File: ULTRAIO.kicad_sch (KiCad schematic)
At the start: 8 parts, among them U6 FDC37C932FR_1.3

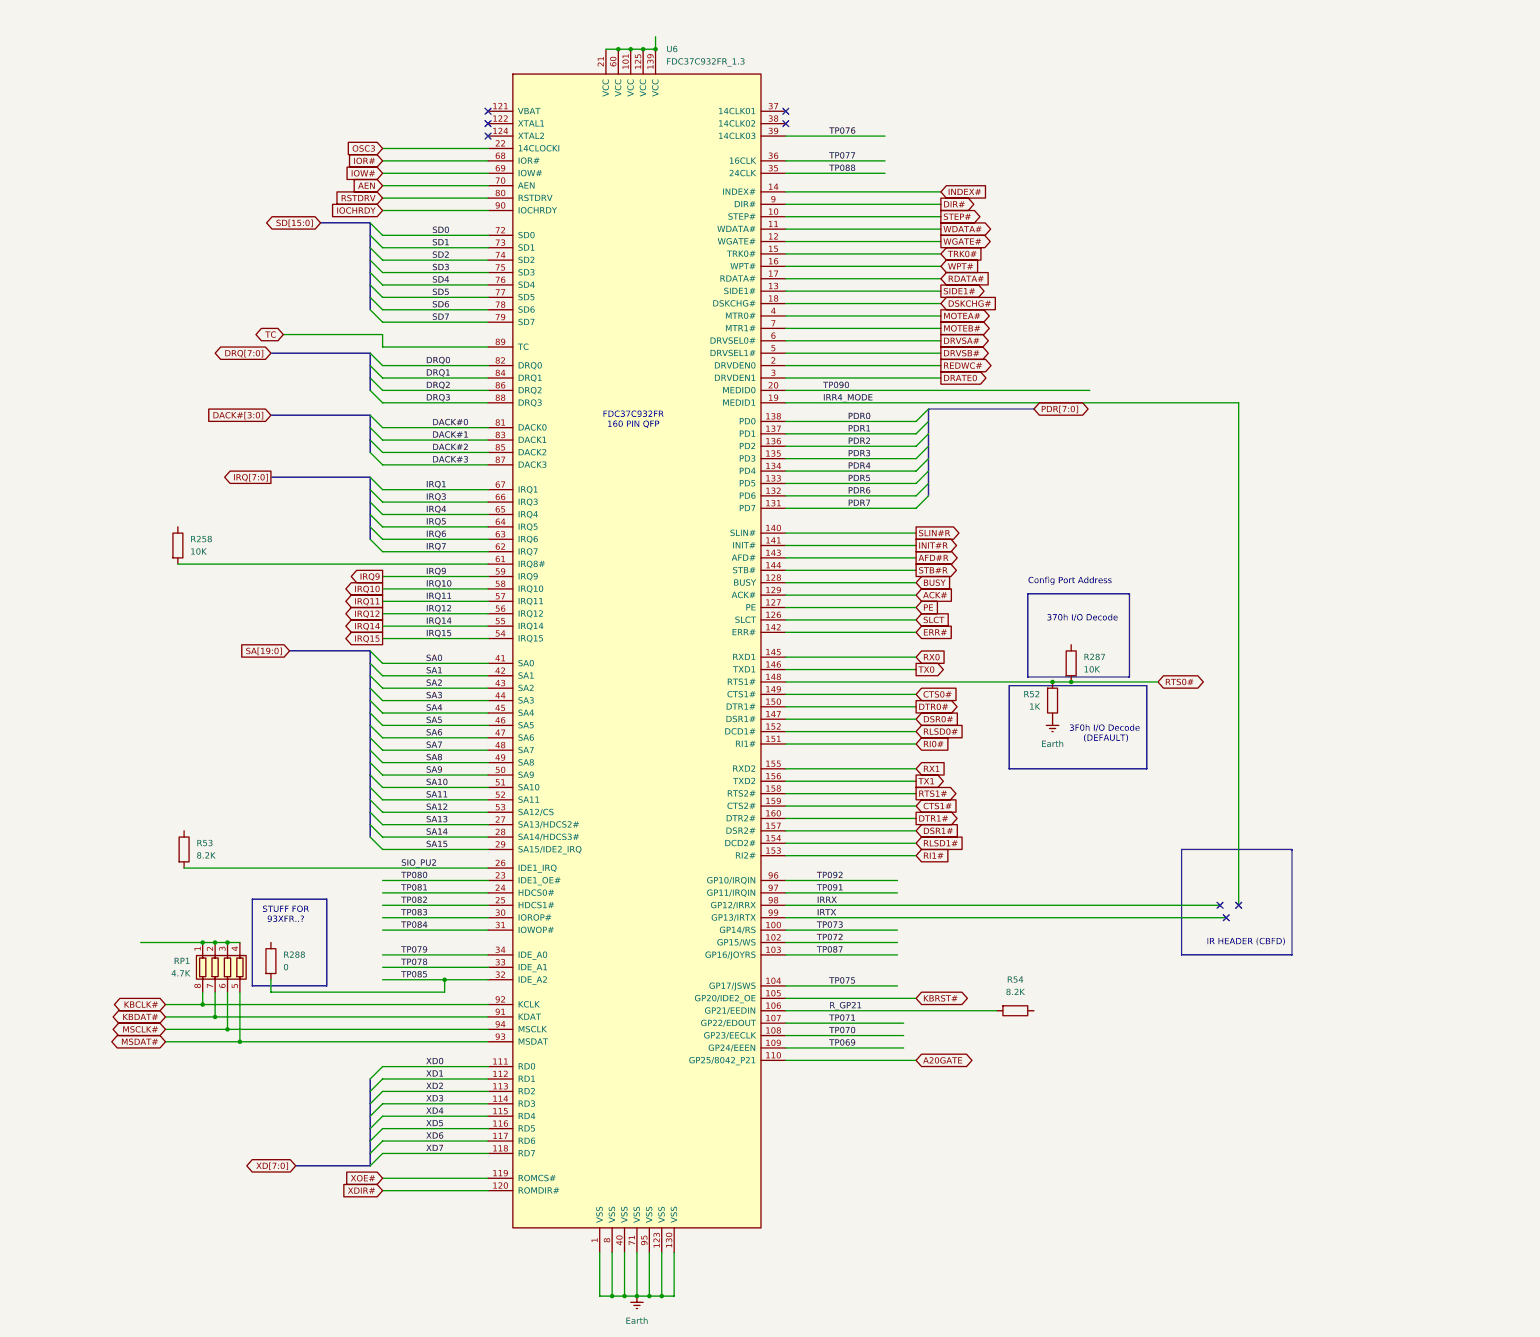
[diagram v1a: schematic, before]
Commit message: ULTRA I/O page 14
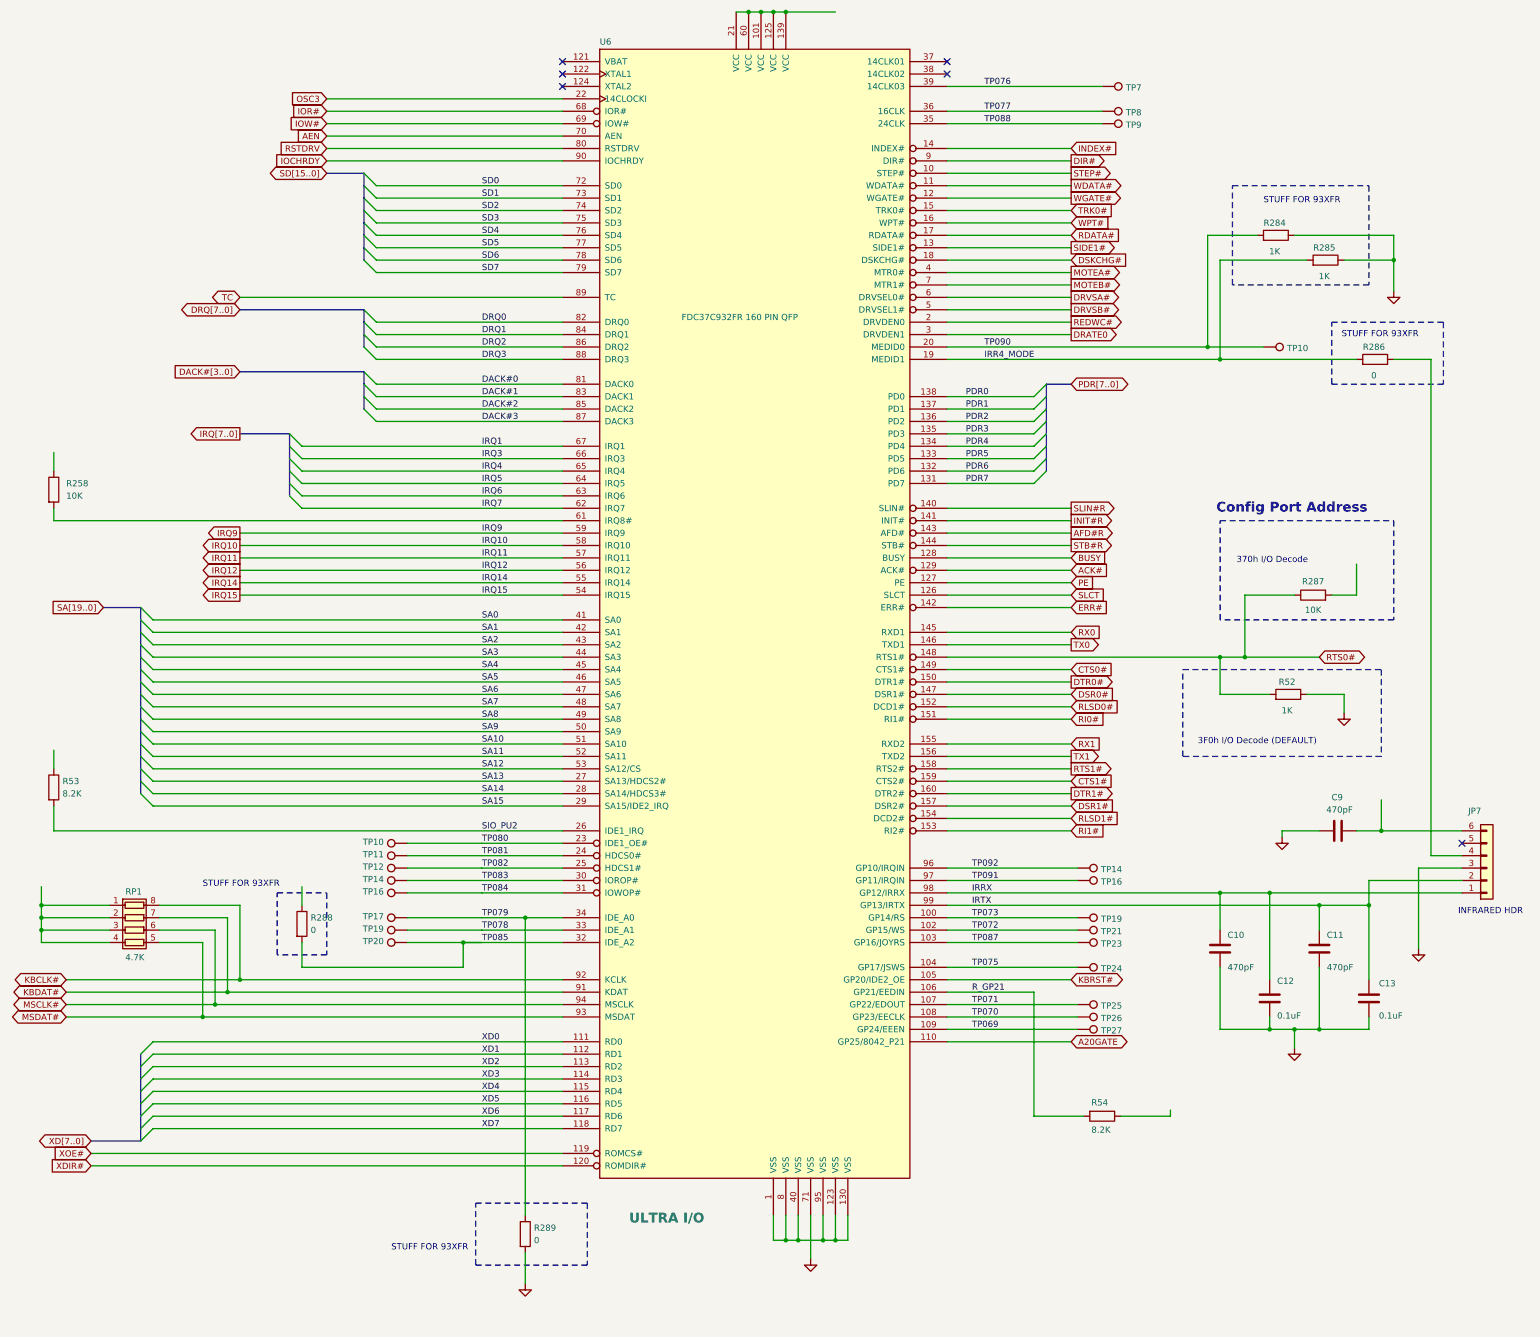
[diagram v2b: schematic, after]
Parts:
- added C10, C11, C9: 470pF, Capacitor_SMD:C_0201_0603Metric, symbol Device:C
- added C12, C13: 0.1uF, Capacitor_SMD:C_0201_0603Metric, symbol Device:C
- added JP7: Conn_01x06, symbol Connector_Generic:Conn_01x06
- added R284, R285: 1K, Resistor_SMD:R_0201_0603Metric, symbol Device:R
- added R286, R289: 0, Resistor_SMD:R_0201_0603Metric, symbol Device:R
- added TP10 (x2), TP11, TP12, TP14 (x2), TP16 (x2), TP17, TP19 (x2), TP20, TP21, TP23, TP24, TP25, TP26, TP27, TP7, TP8, TP9: TestPoint, symbol Connector:TestPoint
- U6: value FDC37C932FR_1.3 -> FDC37C932FR 160 PIN QFP
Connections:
- net IRR4_MODE: now also R285.2, R286.2
- net IRRX: now also C10.1, C12.1, JP7.1 (Pin_1)
- net IRTX: now also C11.1, C13.1, JP7.2 (Pin_2)
- net RTS0#: now also R287.1; no longer R287.2
- net TP069: now also TP27.1
- net TP070: now also TP26.1
- net TP071: now also TP25.1
- net TP072: now also TP21.1
- net TP073: now also TP19.1
- net TP075: now also TP24.1
- net TP076: now also TP7.1
- net TP077: now also TP8.1
- net TP078: now also TP19.1
- net TP079: now also R289.1, TP17.1
- net TP080: now also TP10.1
- net TP081: now also TP11.1
- net TP082: now also TP12.1
- net TP083: now also TP14.1
- net TP084: now also TP16.1
- net TP085: now also TP20.1
- net TP087: now also TP23.1
- net TP088: now also TP9.1
- net TP090: now also R284.2, TP10.1
- net TP091: now also TP16.1
- net TP092: now also TP14.1
- net Earth: no longer names the net of U6.1 (VSS), U6.123 (VSS), U6.130 (VSS), U6.40 (VSS), U6.8 (VSS), U6.95 (VSS)
- net Earth: no longer R52.1, U6.71 (VSS)
- new net: JP7.4 (Pin_4), R286.1
- new net: C9.2, JP7.6 (Pin_6)
- new net GND: C10.2, C11.2, C12.2, C13.2, C9.1, JP7.3 (Pin_3), R284.1, R285.1, R289.2, R52.1, U6.71 (VSS)
- no-connect marks 8 -> 6
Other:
- note added: "INFRARED HDR"
- note added: "STUFF FOR 93XFR"
- note removed: "FDC37C932FR 160 PIN QFP"
- note removed: "IR HEADER (CBFD)"
- note removed: "STUFF FOR 93XFR..?"
- title: (none) -> I/O CONTROLLER (ULTRA I/O)
- moved on the sheet: R258, R287, R288, R52, R53, R54, RP1
